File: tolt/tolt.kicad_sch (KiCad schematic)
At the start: 3 parts, among them J2 USB_C_Receptacle_USB2.0

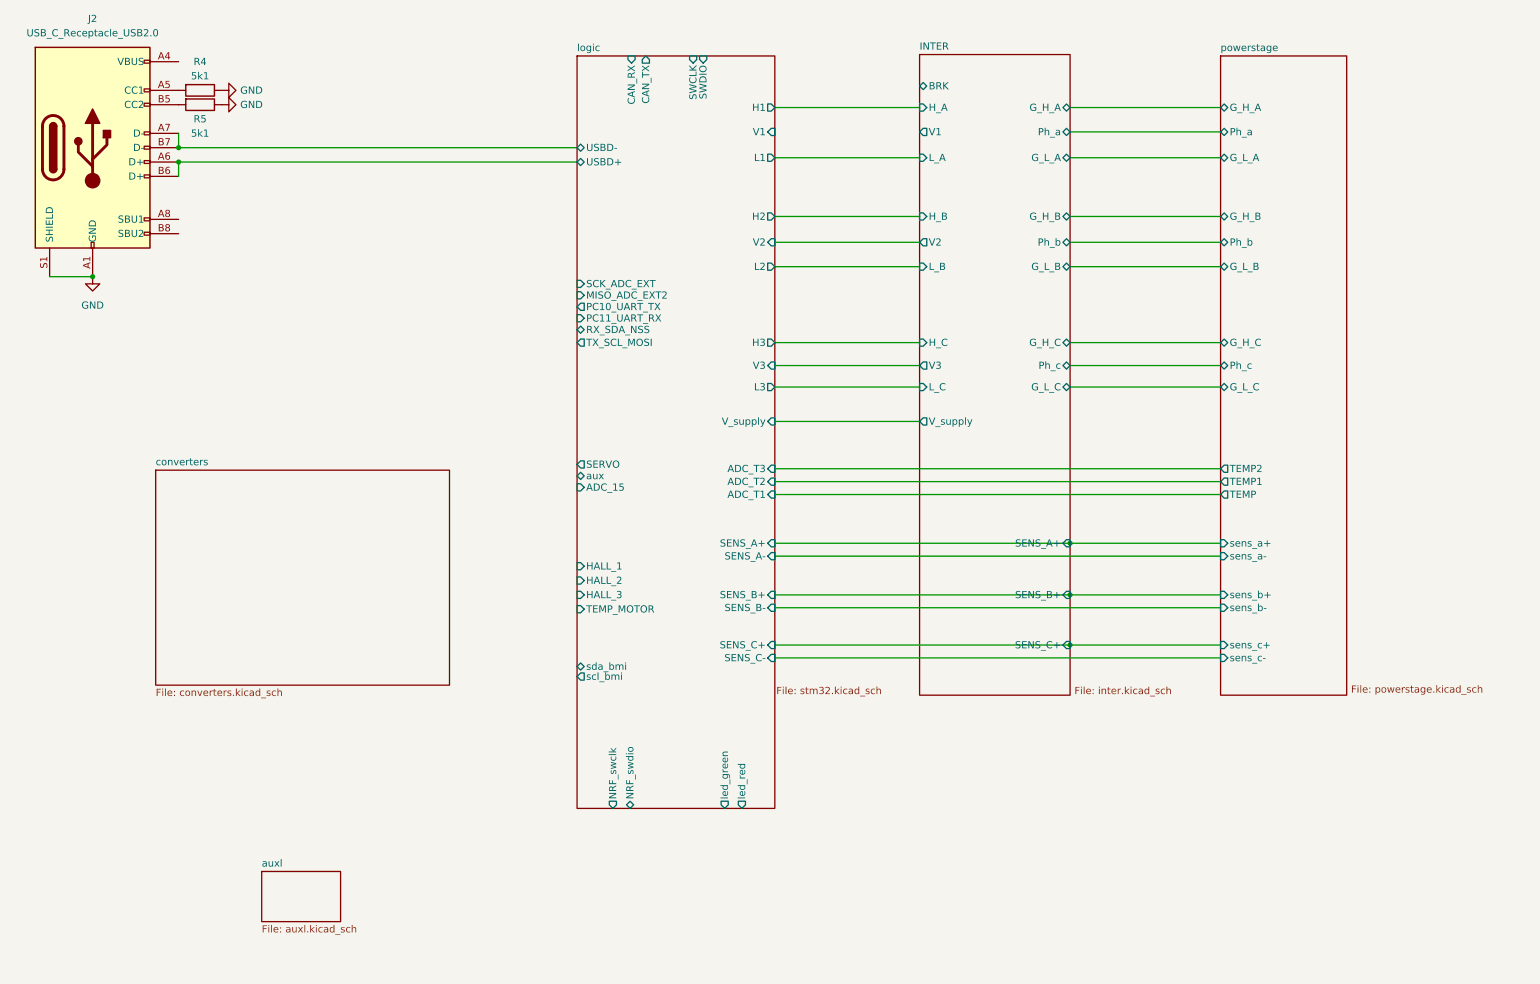
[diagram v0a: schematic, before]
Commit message: Reapply "Merge branch 'main' of https://github.com/LJBoxx/bigtolt"
This reverts commit 10d1035653869a11abcc4dc45a35a471baa73785.
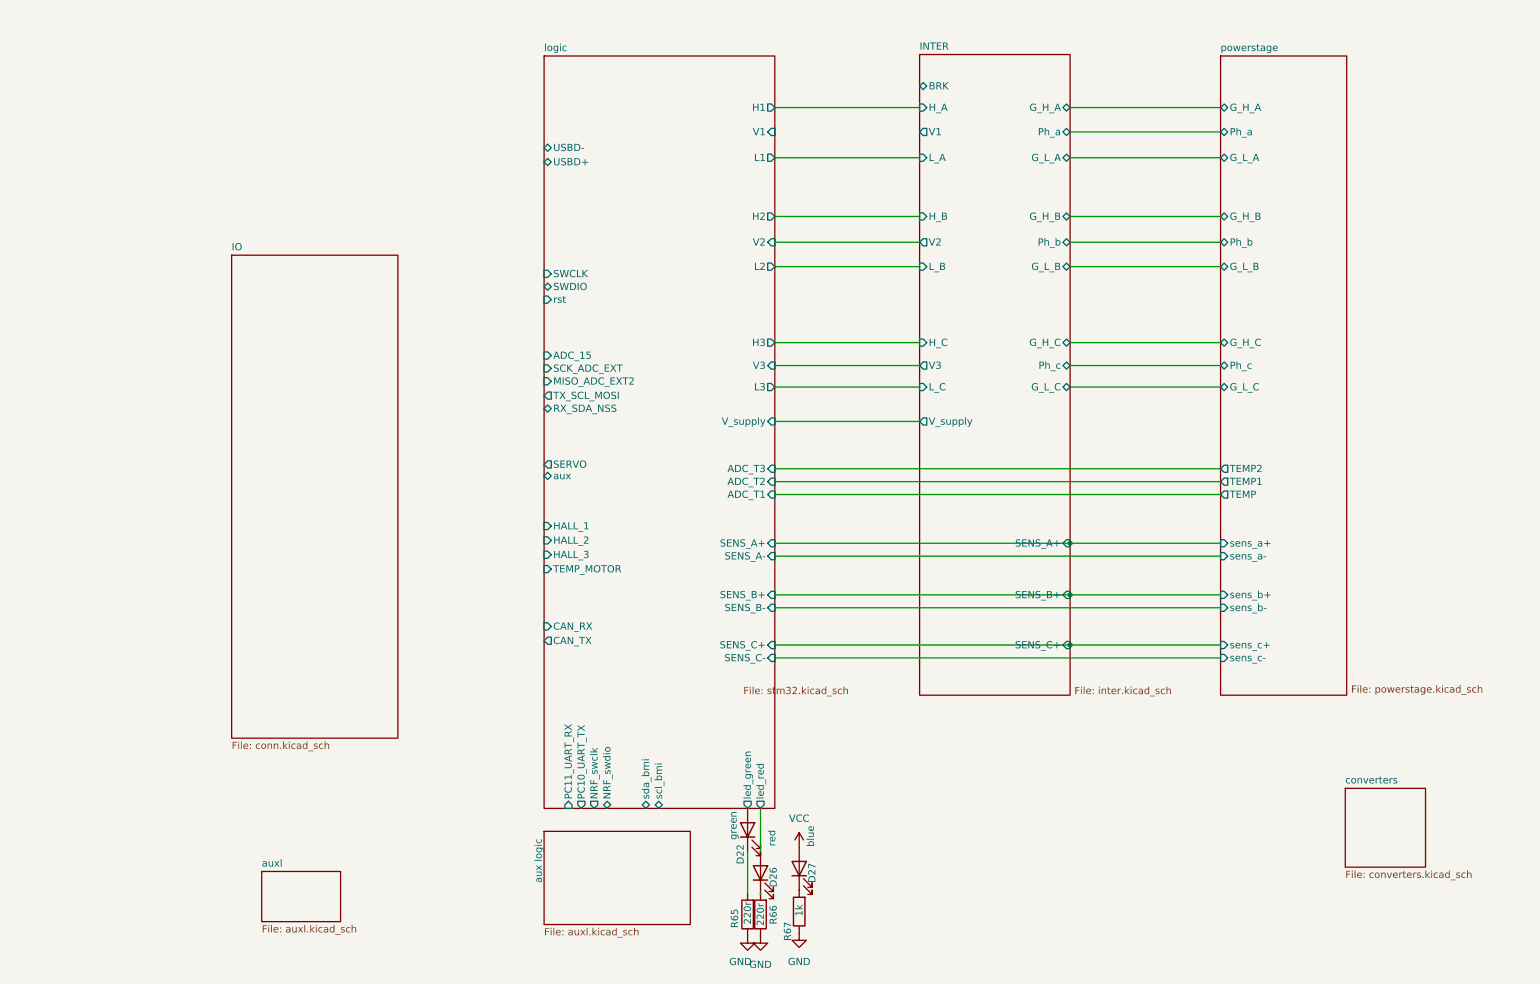
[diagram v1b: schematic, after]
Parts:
- removed J2: USB_C_Receptacle_USB2.0, Connector_USB:USB_C_Receptacle_G-Switch_GT-USB-7051x, symbol Connector:USB_C_Receptacle_USB2.0
- removed R4, R5: 5k1, Resistor_SMD:R_0603_1608Metric, symbol Device:R
- added D22: green, symbol Device:LED
- added D26: red, symbol Device:LED
- added D27: blue, symbol Device:LED
- added R65, R66: 220r, Resistor_SMD:R_0603_1608Metric, symbol Device:R
- added R67: 1k, Resistor_SMD:R_0603_1608Metric, symbol Device:R
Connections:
- net GND: now also R65.1, R66.1, R67.1
- net logic/led_green: now also D22.2 (A)
- net logic/led_red: now also D26.2 (A)
- new net: D27.1 (K), R67.2
- new net: D26.1 (K), R66.2
- new net: D22.1 (K), R65.2
- new net VCC: D27.2 (A)
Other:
- added sheet IO (conn.kicad_sch)
- added sheet aux logic (auxl.kicad_sch)
- sheet logic ports: added rst; removed none
